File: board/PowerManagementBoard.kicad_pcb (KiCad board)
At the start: 2 copper layers, 167.6 x 115.1 mm, 164 parts, among them IC1 ACS37010LLZATR-030B3, IC2 ACS37010LLZATR-030B3, IC3 ACS37010LLZATR-030B3, IC4 ACS37010LLZATR-030B3, IC6 ACS37010LLZATR-030B3, J1 RJ45_LED_Shielded, J10 768250002, J11 768250002, J12 768250002, J13 768250002, J14 768250002, J15 768250002, J16 768250002, J17 768250002, J18 768250002, J2 SS-73100-082, J3 SS-73100-082, J5 768250002, J6 768250002, J7 768250002, J8 768250002, J9 768250002, Q1 BSS138, Q2 IPB180N10S4-02, Q3 Si4162DY, Q4 IPB180N10S4-02, Q5 Si4162DY, Q6 Si4162DY, Q7 Si4162DY, Q8 Si4162DY, Q9 IPB180N10S4-02, U1 LT1910, U10 ACS72981LLRATR-100U3, U11 LT1910, U12 LT1910, U13 LT1910, U14 LT1910, U15 Teensy4.1_DEV-16771, U16 OKI-78SR-3.3_1.5-W36H-C, U17 OKI-78SR-5_1.5-W36H-C, U19 LT1910, U2 LM5050MK-1_NOPB, U3 LM5050MK-1_NOPB, U4 Opamp_Dual, U5 Opamp_Dual, U6 Opamp_Dual

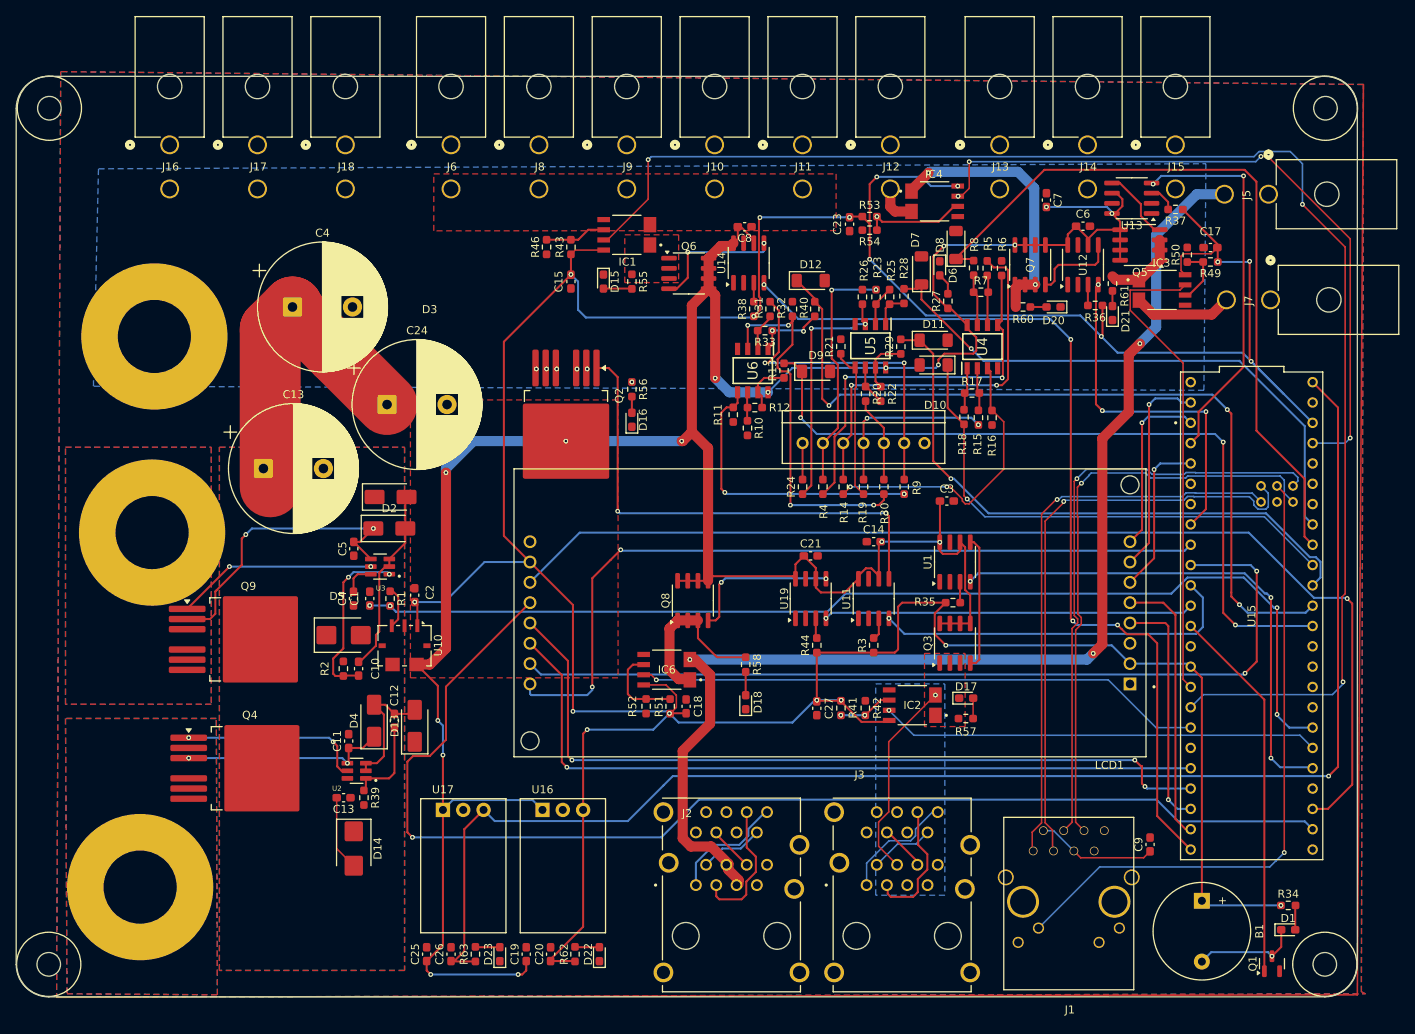
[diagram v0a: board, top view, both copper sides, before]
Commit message: experimented with layout
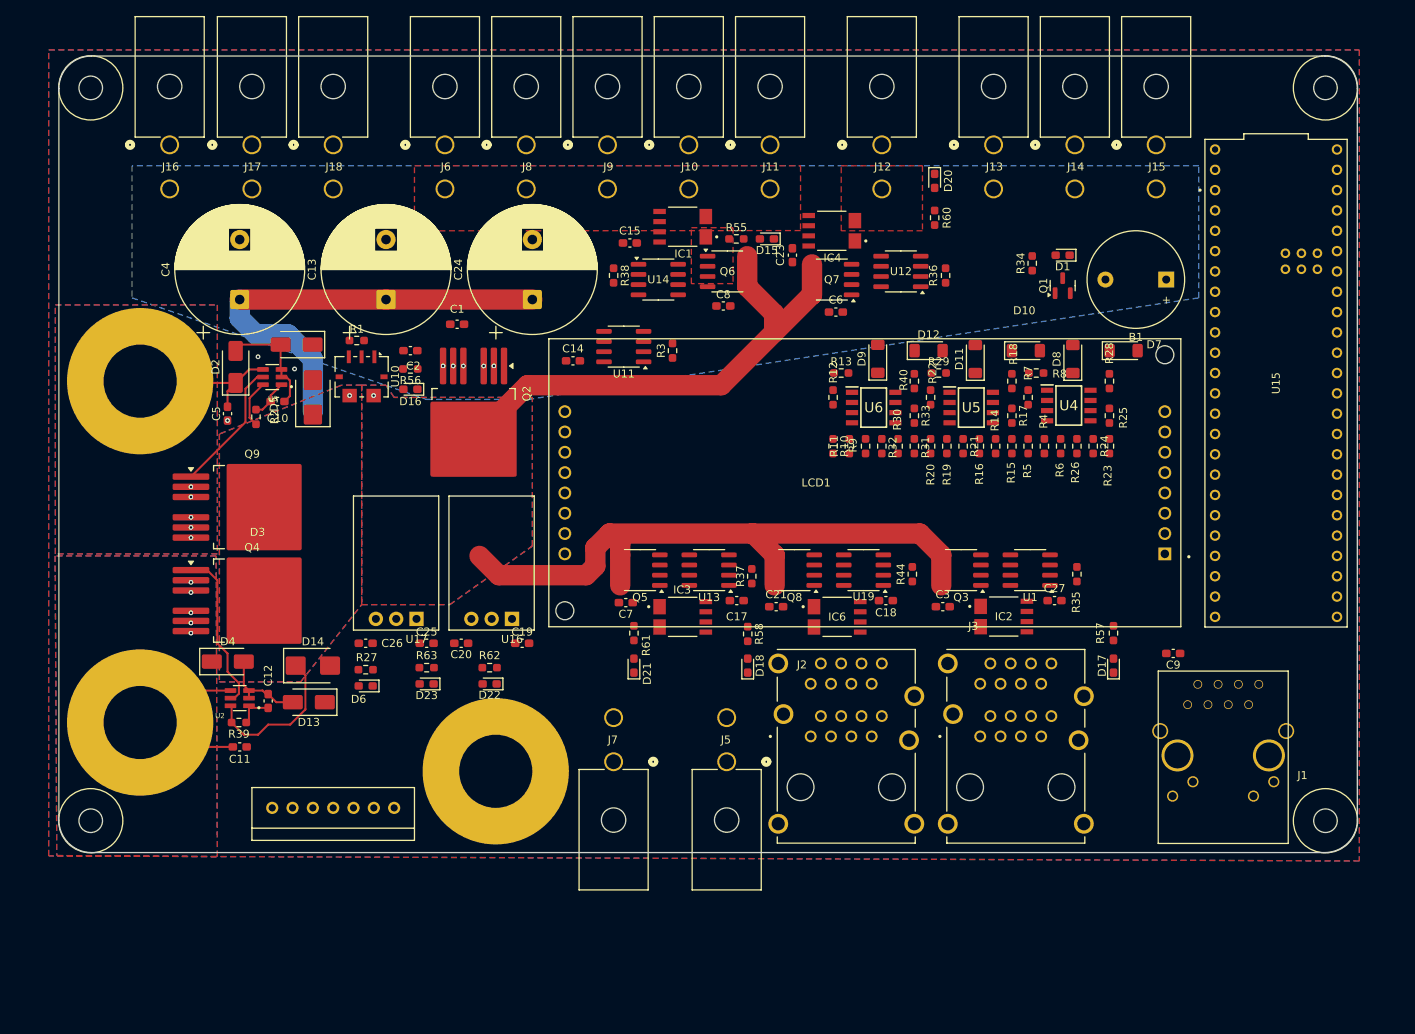
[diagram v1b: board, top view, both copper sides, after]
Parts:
- removed the C13 at (75.0, 122.2)
- removed the C4 at (76.2, 97.3)
- removed R41, R42, R43, R46, R49, R50, R51, R52, R53, R54: 10k, Resistor_SMD:R_0603_1608Metric_Pad0.98x0.95mm_HandSolder
- moved J7 100.4 mm to (108.7, 117.7), turned to 0 degrees
- moved J5 98.1 mm to (122.8, 117.7), turned to 0 degrees
- moved D1 88.9 mm to (164.8, 54.4), turned to 180 degrees
- moved D6 88.7 mm to (77.7, 108.2), turned to 180 degrees
- moved Q1 88.7 mm to (164.8, 58.2)
- moved R34 86.4 mm to (161.0, 55.4), turned to 90 degrees
- moved R27 86.1 mm to (77.7, 106.2), turned to 180 degrees
- moved B1 77.8 mm to (177.8, 57.4), turned to 180 degrees
- moved Q5 74.5 mm to (112.0, 93.7)
- moved D21 74.3 mm to (111.3, 105.7)
- moved R61 74.1 mm to (111.3, 101.6)
- moved C17 73.8 mm to (124.1, 97.5), turned to 0 degrees
- moved C7 72.8 mm to (110.2, 97.8), turned to 180 degrees
- moved IC3 72.5 mm to (117.3, 99.6)
- moved U13 70.4 mm to (120.7, 93.7)
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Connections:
- net Net-(D14-K) renamed /Current Protection/Batt_to_CS
- net Net-(D2-K) renamed /Current Protection/Batt2
- net Net-(D4-K) renamed /Current Protection/Batt1
- IC1 pad 6: Net-(IC1-VREF) -> unconnected-(IC1-VREF-Pad6)
- IC2 pad 6: Net-(IC2-VREF) -> unconnected-(IC2-VREF-Pad6)
- IC3 pad 6: Net-(IC3-VREF) -> unconnected-(IC3-VREF-Pad6)
- IC4 pad 6: Net-(IC4-VREF) -> unconnected-(IC4-VREF-Pad6)
- IC6 pad 6: Net-(IC6-VREF) -> unconnected-(IC6-VREF-Pad6)
- R10 pad 1: Net-(U6B--) -> Net-(U6A--)
- R11 pad 1: Net-(U6B-+) -> Net-(U6A-+)
- R12 pad 2: Net-(U6B--) -> Net-(U6A--)
- R14 pad 1: Net-(U4A-+) -> Net-(U5B-+)
- R15 pad 1: Net-(U4A--) -> Net-(U5B--)
- R16 pad 1: Net-(U4A-+) -> Net-(U5B-+)
- R17 pad 2: Net-(U4A--) -> Net-(U5B--)
- R19 pad 1: Net-(U5B-+) -> Net-(U5A-+)
- R20 pad 1: Net-(U5B--) -> Net-(U5A--)
- R21 pad 1: Net-(U5B-+) -> Net-(U5A-+)
- R22 pad 2: Net-(U5B--) -> Net-(U5A--)
- R23 pad 1: Net-(U5A--) -> Net-(U4B--)
- R24 pad 1: Net-(U5A-+) -> Net-(U4B-+)
- R25 pad 2: Net-(U5A--) -> Net-(U4B--)
- R26 pad 1: Net-(U5A-+) -> Net-(U4B-+)
- R30 pad 1: Net-(U6A-+) -> Net-(U6B-+)
- R31 pad 1: Net-(U6A--) -> Net-(U6B--)
- R32 pad 1: Net-(U6A-+) -> Net-(U6B-+)
- R33 pad 2: Net-(U6A--) -> Net-(U6B--)
- R4 pad 1: Net-(U4B-+) -> Net-(U4A-+)
- R5 pad 1: Net-(U4B--) -> Net-(U4A--)
- R6 pad 1: Net-(U4B-+) -> Net-(U4A-+)
- R7 pad 2: Net-(U4B--) -> Net-(U4A--)
- R9 pad 1: Net-(U6B-+) -> Net-(U6A-+)
- U15 pad 10: /Switching Circuit/M9_EN -> unconnected-(U15-CS1-Pad10)
- U15 pad 27: /TeensyandEthernetCircuit/CSensem5 -> unconnected-(U15-A13-Pad27)
- U15 pad 3.3V_1: +3V3 -> unconnected-(U15-3.3V-Pad3.3V_1)
- U15 pad 3.3V_2: +3V3 -> unconnected-(U15-3.3V-Pad3.3V_1)_1
- U15 pad 36: unconnected-(U15-CS2-Pad36) -> /Switching Circuit/M9_EN
- U4 pad 1: Net-(R17-Pad1) -> Net-(R7-Pad1)
- U4 pad 7: Net-(R7-Pad1) -> Net-(R25-Pad1)
- U5 pad 1: Net-(R25-Pad1) -> Net-(R22-Pad1)
- U5 pad 7: Net-(R22-Pad1) -> Net-(R17-Pad1)
- U6 pad 1: Net-(R33-Pad1) -> Net-(R12-Pad1)
- U6 pad 7: Net-(R12-Pad1) -> Net-(R33-Pad1)
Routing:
- net +3V3: track 475.6 -> 0.00 mm, vias 19 -> 0
- net +24V: track 358.5 -> 146.4 mm, vias 17 -> 1
- net +5V: track 183.5 -> 0.00 mm, vias 1 -> 0
- net /Current-Sensinator/LCVout: track 183.2 -> 0.00 mm, vias 3 -> 0
- net /LCD/D6: track 153.2 -> 0.00 mm, vias 1 -> 0
- net /Current-Sensinator/m9out: track 152.8 -> 0.00 mm, vias 3 -> 0
- net /LCD/D7: track 137.8 -> 0.00 mm, vias 1 -> 0
- net /Current Protection/BattVout: track 135.7 -> 0.00 mm, vias 4 -> 0
- net /Switching Circuit/LC_EN: track 115.7 -> 0.00 mm, vias 4 -> 0
- net /LCD/D3: track 111.9 -> 0.00 mm, vias 2 -> 0
- net /TeensyandEthernetCircuit/CellSense2: track 103.4 -> 0.00 mm, vias 3 -> 0
- net /LCD/D2: track 100.0 -> 0.00 mm, vias 2 -> 0
- net /LCD/D5: track 99.4 -> 0.00 mm, vias 3 -> 0
- net /TeensyandEthernetCircuit/CellSense1: track 95.8 -> 0.00 mm, vias 3 -> 0
- net /LCD/D4: track 95.4 -> 0.00 mm, vias 1 -> 0
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- added copper zone on B.Cu, net +24V
- added copper zone on F.Cu, net /Anderson/AUX
- removed copper zone on F.Cu, net /Current-Sensinator/m2in
- removed copper zone on B.Cu, net /Current-Sensinator/m2out
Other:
- board size 167.6 x 115.1 mm -> 162.3 x 99.6 mm
